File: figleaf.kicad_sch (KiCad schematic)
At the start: 72 parts, among them J1 Conn_01x02_Pin, J2 HRO_TYPE-C-31-M-14, J3 Battery, J9 TC2030_SWD, Q2 2N7002, SW1 PWR, SW2 RST, U1 SRV05-4, U10 MAX17048, U3 BQ24075, U8 nRF52840_moko_mk08

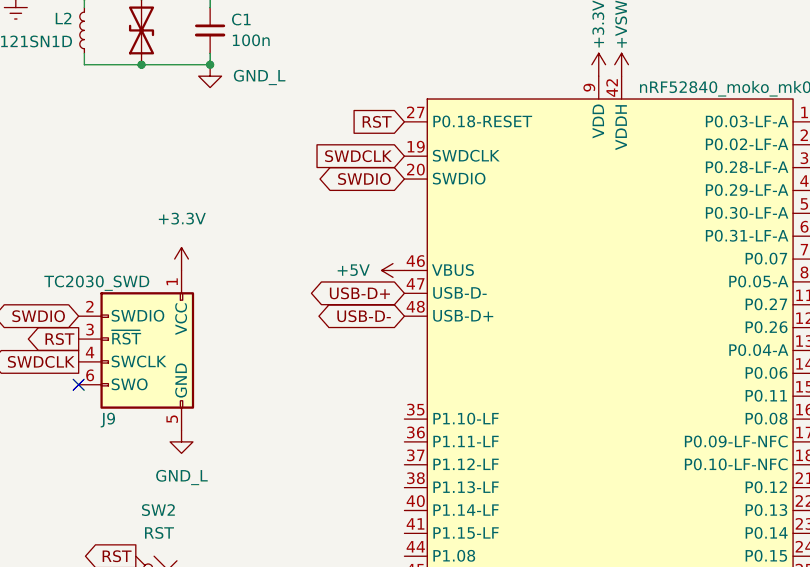
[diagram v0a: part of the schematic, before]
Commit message: pre right side
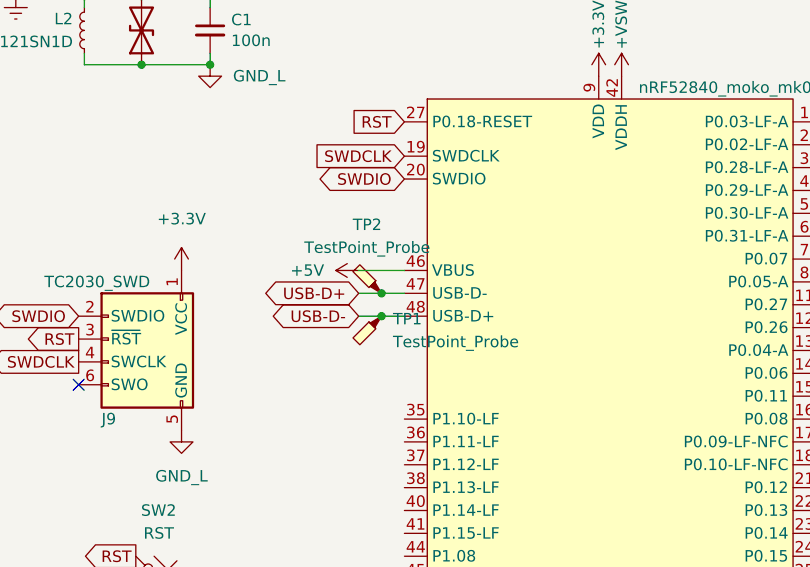
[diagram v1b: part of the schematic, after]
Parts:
- added TP1, TP2: TestPoint_Probe, TestPoint:TestPoint_Pad_D1.0mm, symbol Connector:TestPoint_Probe
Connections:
- net USB-D+: now also TP2.1
- net USB-D-: now also TP1.1
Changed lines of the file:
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@@
 	)
 	(junction
+		(at 67.31 101.6)
+		(diameter 0)
+		(color 0 0 0 0)
+	)
+	(junction
 		(at 93.98 158.75)
 		(diameter 0)
@@
 	)
 	(junction
+		(at 67.31 104.14)
+		(diameter 0)
+		(color 0 0 0 0)
+	)
+	(junction
 		(at 49.53 29.21)
 		(diameter 0)
@@
 	(wire
 		(pts
+			(xy 67.31 104.14) (xy 69.85 104.14)
+		)
+		(stroke
+			(width 0)
+			(type default)
+		)
+	)
+	(wire
+		(pts
 			(xy 349.25 142.24) (xy 354.33 142.24)
 		)
@@
 	(wire
 		(pts
+			(xy 64.77 99.06) (xy 69.85 99.06)
+		)
+		(stroke
+			(width 0)
+			(type default)
+		)
+	)
+	(wire
+		(pts
 			(xy 49.53 29.21) (xy 55.88 29.21)
 		)
@@
 	(wire
 		(pts
+			(xy 67.31 101.6) (xy 69.85 101.6)
+		)
+		(stroke
+			(width 0)
+			(type default)
+		)
+	)
+	(wire
+		(pts
 			(xy 313.69 127) (xy 313.69 132.08)
 		)
@@
 	(wire
 		(pts
+			(xy 64.77 104.14) (xy 67.31 104.14)
+		)
+		(stroke
+			(width 0)
+			(type default)
+		)
+	)
+	(wire
+		(pts
 			(xy 262.89 152.4) (xy 262.89 157.48)
 		)
@@
 	(wire
 		(pts
+			(xy 64.77 101.6) (xy 67.31 101.6)
+		)
+		(stroke
+			(width 0)
+			(type default)
+		)
+	)
+	(wire
+		(pts
 			(xy 267.97 127) (xy 267.97 132.08)
 		)
@@
 	(global_label "USB-D+"
 		(shape bidirectional)
-		(at 69.85 101.6 180)
+		(at 64.77 101.6 180)
 		(fields_autoplaced yes)
 		(effects
@@
 		)
 		(property "Intersheetrefs" "${INTERSHEET_REFS}"
-			(at 59.2121 101.6794 0)
+			(at 54.1321 101.6794 0)
 			(effects
 				(font
@@
 	(global_label "USB-D-"
 		(shape bidirectional)
-		(at 69.85 104.14 180)
+		(at 64.77 104.14 180)
 		(fields_autoplaced yes)
 		(effects
@@
 		)
 		(property "Intersheetrefs" "${INTERSHEET_REFS}"
-			(at 59.2121 104.2194 0)
+			(at 54.1321 104.2194 0)
 			(effects
 				(font
@@
 	)
 	(symbol
+		(lib_id "Connector:TestPoint_Probe")
+		(at 67.31 101.6 90)
+		(unit 1)
+		(exclude_from_sim no)
+		(in_bom yes)
+		(on_board yes)
+		(dnp no)
+		(fields_autoplaced yes)
+		(property "Reference" "TP2"
+			(at 65.7225 93.98 90)
+			(effects
+				(font
+					(size 1.27 1.27)
+				)
+			)
+		)
+		(property "Value" "TestPoint_Probe"
+			(at 65.7225 96.52 90)
+			(effects
+				(font
+					(size 1.27 1.27)
+				)
+			)
+		)
+		(property "Footprint" "TestPoint:TestPoint_Pad_D1.0mm"
+			(at 67.31 96.52 0)
+			(effects
+				(font
+					(size 1.27 1.27)
+				)
+				(hide yes)
+			)
+		)
+		(property "Datasheet" "~"
+			(at 67.31 96.52 0)
+			(effects
+				(font
+					(size 1.27 1.27)
+				)
+				(hide yes)
+			)
+		)
+		(property "Description" "test point (alternative probe-style design)"
+			(at 67.31 101.6 0)
+			(effects
+				(font
+					(size 1.27 1.27)
+				)
+				(hide yes)
+			)
+		)
+		(pin "1"
+		)
+		(instances
+			(project "figleaf"
+				(path "/49b93484-acc8-4f70-93bc-7a6072a35fe8"
+					(reference "TP2")
+					(unit 1)
+				)
+			)
+		)
+	)
+	(symbol
 		(lib_id "power:GND")
 		(at 344.17 106.68 180)
@@
 	)
 	(symbol
+		(lib_id "Connector:TestPoint_Probe")
+		(at 67.31 104.14 180)
+		(unit 1)
+		(exclude_from_sim no)
+		(in_bom yes)
+		(on_board yes)
+		(dnp no)
+		(fields_autoplaced yes)
+		(property "Reference" "TP1"
+			(at 68.58 104.4574 0)
+			(effects
+				(font
+					(size 1.27 1.27)
+				)
+				(justify right)
+			)
+		)
+		(property "Value" "TestPoint_Probe"
+			(at 68.58 106.9974 0)
+			(effects
+				(font
+					(size 1.27 1.27)
+				)
+				(justify right)
+			)
+		)
+		(property "Footprint" "TestPoint:TestPoint_Pad_D1.0mm"
+			(at 62.23 104.14 0)
+			(effects
+				(font
+					(size 1.27 1.27)
+				)
+				(hide yes)
+			)
+		)
+		(property "Datasheet" "~"
+			(at 62.23 104.14 0)
+			(effects
+				(font
+					(size 1.27 1.27)
+				)
+				(hide yes)
+			)
+		)
+		(property "Description" "test point (alternative probe-style design)"
+			(at 67.31 104.14 0)
+			(effects
+				(font
+					(size 1.27 1.27)
+				)
+				(hide yes)
+			)
+		)
+		(pin "1"
+		)
+		(instances
+			(project ""
+				(path "/49b93484-acc8-4f70-93bc-7a6072a35fe8"
+					(reference "TP1")
+					(unit 1)
+				)
+			)
+		)
+	)
+	(symbol
 		(lib_id "0_graz_symbols:SW_OKM")
 		(at 288.29 116.84 0)
@@
 	(symbol
 		(lib_id "power:+5V")
-		(at 69.85 99.06 90)
+		(at 64.77 99.06 90)
 		(unit 1)
 		(exclude_from_sim no)
@@
 		(dnp no)
 		(property "Reference" "#PWR051"
-			(at 73.66 99.06 0)
+			(at 68.58 99.06 0)
 			(effects
 				(font
@@
 		)
 		(property "Value" "+5V"
-			(at 64.135 99.06 90)
+			(at 59.055 99.06 90)
 			(effects
 				(font
@@
 		)
 		(property "Footprint" ""
-			(at 69.85 99.06 0)
+			(at 64.77 99.06 0)
 			(effects
 				(font
@@
 		)
 		(property "Datasheet" ""
-			(at 69.85 99.06 0)
+			(at 64.77 99.06 0)
 			(effects
 				(font
@@
 		)
 		(property "Description" "Power symbol creates a global label with name \"+5V\""
-			(at 69.85 99.06 0)
+			(at 64.77 99.06 0)
 			(effects
 				(font
